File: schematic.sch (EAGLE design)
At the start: 32 parts, among them Q3 IRF540

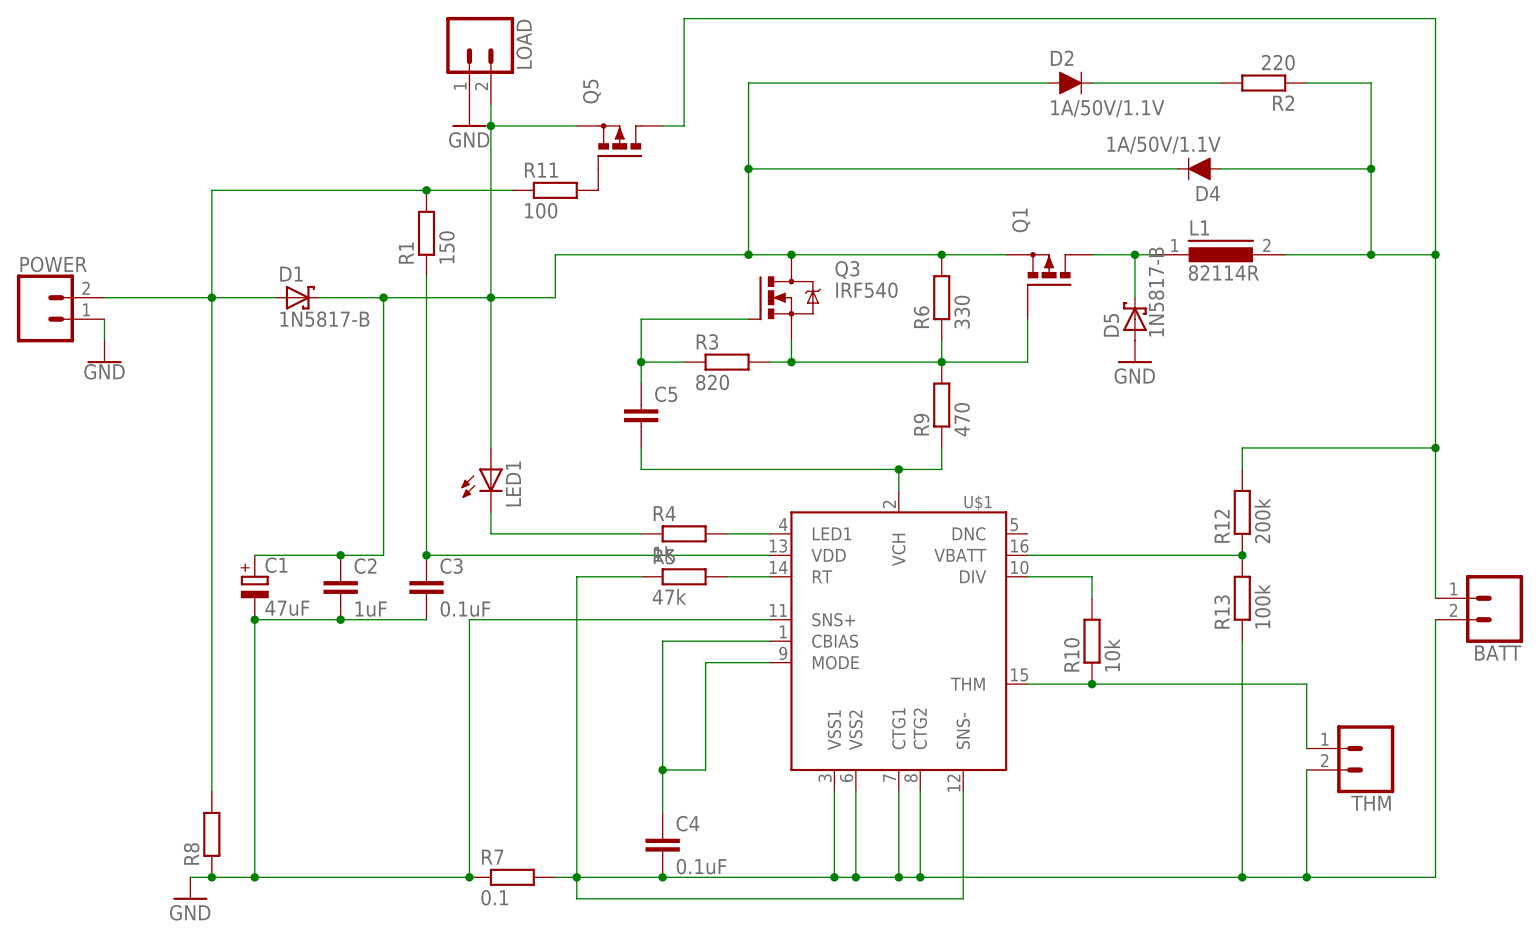
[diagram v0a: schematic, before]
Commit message: Layout done
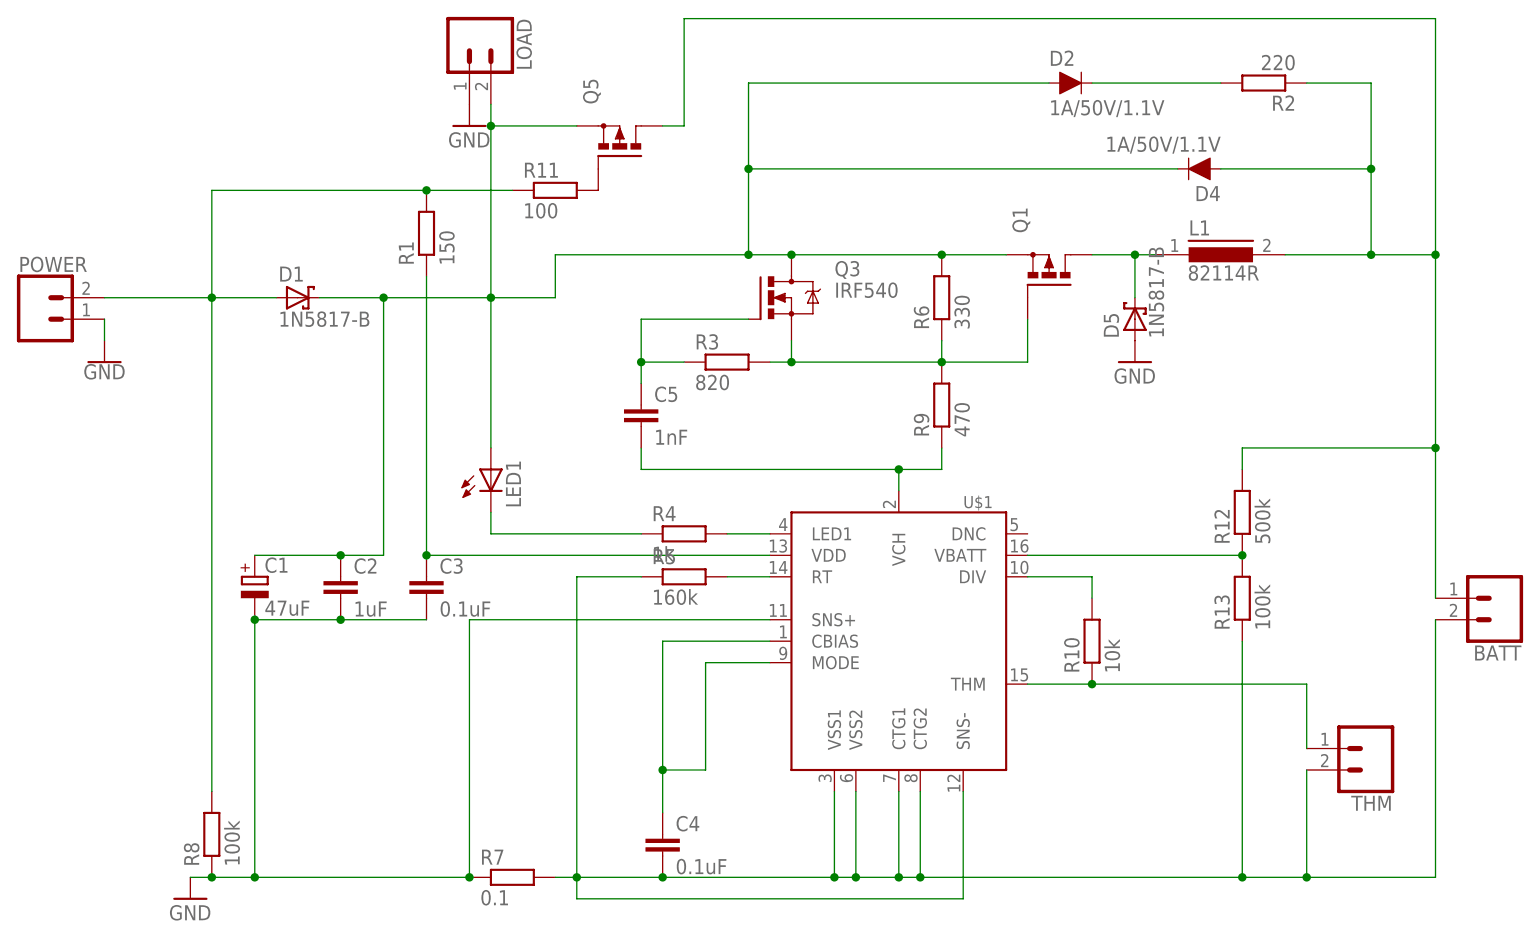
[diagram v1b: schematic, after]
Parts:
- C5: value (none) -> 1nF
- R12: value 200k -> 500k
- R5: value 47k -> 160k
- R8: value (none) -> 100k
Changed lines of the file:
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@@
 <part name="R4" library="rcl" library_urn="urn:adsk.eagle:library:334" deviceset="R-EU_" device="0207/10" value="1k"/>
 <part name="R10" library="rcl" library_urn="urn:adsk.eagle:library:334" deviceset="R-EU_" device="0207/10" value="10k"/>
-<part name="R12" library="rcl" library_urn="urn:adsk.eagle:library:334" deviceset="R-EU_" device="0207/10" value="200k"/>
+<part name="R12" library="rcl" library_urn="urn:adsk.eagle:library:334" deviceset="R-EU_" device="0207/10" value="500k"/>
 <part name="R13" library="rcl" library_urn="urn:adsk.eagle:library:334" deviceset="R-EU_" device="0207/10" value="100k"/>
 <part name="R7" library="rcl" library_urn="urn:adsk.eagle:library:334" deviceset="R-EU_" device="0207/10" value="0.1"/>
-<part name="R8" library="rcl" library_urn="urn:adsk.eagle:library:334" deviceset="R-EU_" device="0207/10"/>
+<part name="R8" library="rcl" library_urn="urn:adsk.eagle:library:334" deviceset="R-EU_" device="0207/10" value="100k"/>
 <part name="C2" library="rcl" library_urn="urn:adsk.eagle:library:334" deviceset="C-EU" device="025-025X050" value="1uF"/>
 <part name="C3" library="rcl" library_urn="urn:adsk.eagle:library:334" deviceset="C-EU" device="025-025X050" value="0.1uF"/>
@@
 <part name="GND3" library="supply1" library_urn="urn:adsk.eagle:library:371" deviceset="GND" device=""/>
 <part name="GND4" library="supply1" library_urn="urn:adsk.eagle:library:371" deviceset="GND" device=""/>
-<part name="C5" library="rcl" library_urn="urn:adsk.eagle:library:334" deviceset="C-EU" device="025-025X050"/>
-<part name="R5" library="rcl" library_urn="urn:adsk.eagle:library:334" deviceset="R-EU_" device="0207/10" value="47k"/>
+<part name="C5" library="rcl" library_urn="urn:adsk.eagle:library:334" deviceset="C-EU" device="025-025X050" value="1nF"/>
+<part name="R5" library="rcl" library_urn="urn:adsk.eagle:library:334" deviceset="R-EU_" device="0207/10" value="160k"/>
 <part name="Q1" library="transistor-power" library_urn="urn:adsk.eagle:library:400" deviceset="PMOSFET_P" device="TO220BV"/>
 <part name="D1" library="diode" library_urn="urn:adsk.eagle:library:210" deviceset="1N581*" device="" technology="7-B"/>
